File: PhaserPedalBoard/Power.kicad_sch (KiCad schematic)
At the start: 17 parts, among them J1 Footswitch, J7 PowerJack, U1 LMR62014XMF, U4 AMS1117

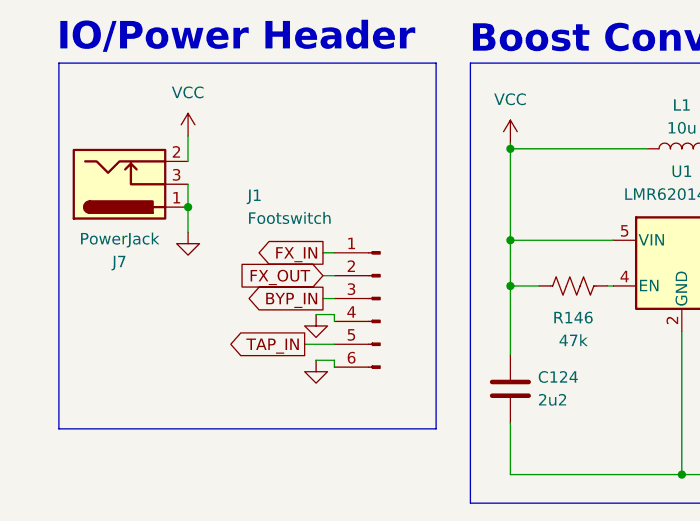
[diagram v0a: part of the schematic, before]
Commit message: DAC stage looks good in sim
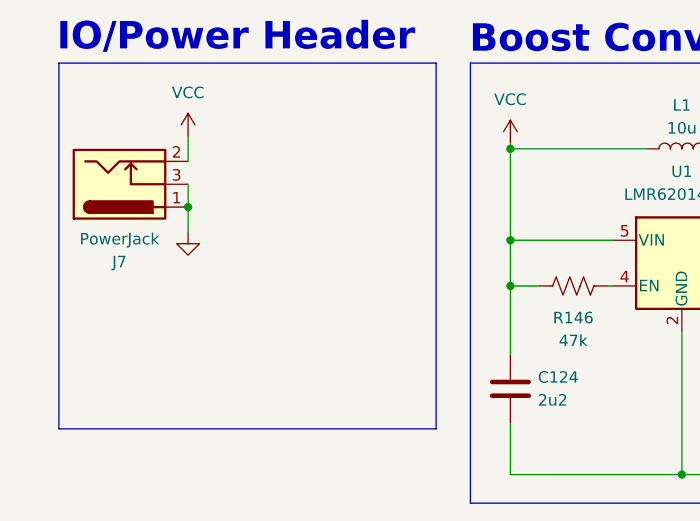
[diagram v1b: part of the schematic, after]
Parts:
- removed J1: Footswitch, symbol Connector:Conn_01x06_Pin
